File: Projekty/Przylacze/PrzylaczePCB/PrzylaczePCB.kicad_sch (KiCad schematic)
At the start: 46 parts, among them J1 Conn_02x20_Odd_Even, J2 USB_B, J3 Conn_01x06, J4 Conn_02x04_Odd_Even, J5 Screw_Terminal_01x06, Q3 2N7002, Q4 2N3904, Q5 2N3904, Q6 2N7002, SW1 SW_Push, U10 74AHC1G04, U11 74AHC1G04, U2 ATSAM4S2AA-AU, U6 NE5532P, U7 LDL1117S33R, U8 DI78M05UAB, U9 TLV3202AID

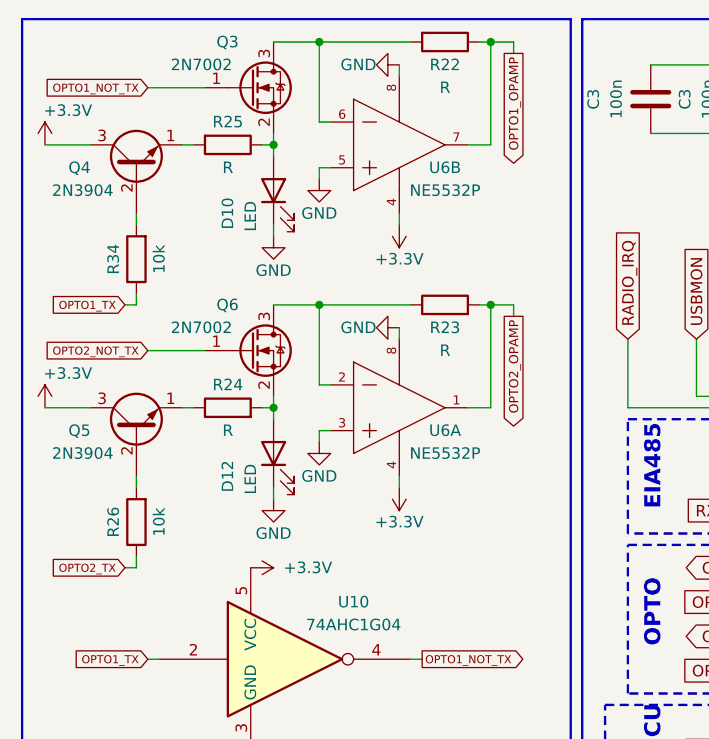
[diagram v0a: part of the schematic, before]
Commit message: PeCeBe wersja Final Omega Prime Ultimate Fatality
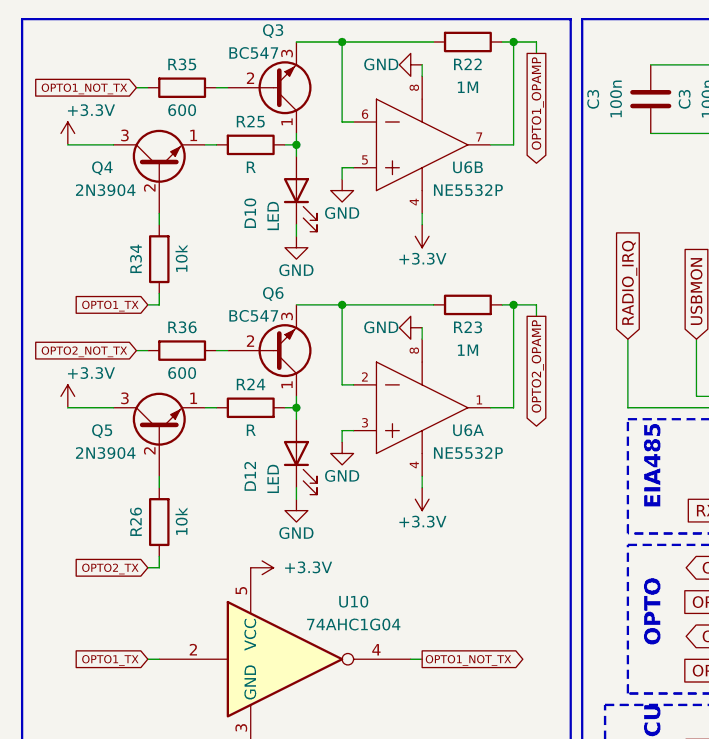
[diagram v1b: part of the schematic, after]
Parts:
- removed Q3, Q6: 2N7002, Package_TO_SOT_SMD:SOT-23, symbol Transistor_FET:2N7002
- added Q3, Q6: BC547, Package_TO_SOT_THT:TO-92_Inline, symbol Transistor_BJT:BC547
- added R35, R36: 600, Resistor_THT:R_Axial_DIN0207_L6.3mm_D2.5mm_P10.16mm_Horizontal, symbol Device:R
- R22, R23: value R -> 1M
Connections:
- net OPTO1_NOT_TX: now also R35.2
- net OPTO2_NOT_TX: now also R36.2
- net at D12.2 (A), R24.2: now also Q6.1 (C)
- net at D10.2 (A), R25.1: now also Q3.1 (C)
- net at R22.2, U6.6 (IN2-): now also Q3.3 (E)
- net at R23.1, U6.2 (IN1-): now also Q6.3 (E)
- new net: Q6.2 (B), R36.1
- new net: Q3.2 (B), R35.1
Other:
- moved on the sheet: D10, D12, Q4, Q5, R22, R23, R24, R25, R26, R34, U6A, U6B
